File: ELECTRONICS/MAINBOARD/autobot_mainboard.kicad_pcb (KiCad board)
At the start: 4 copper layers, 268 x 112 mm, 164 parts, among them IC1 DW3210, J1 USB_C_Receptacle_USB2.0_16P, J10 Conn_01x05_Socket, J11 Conn_01x01_Socket, J12 Conn_01x02_Pin, J13 Conn_01x01_Socket, J17 Conn_01x02_Pin, J18 Conn_01x02_Pin, J19 Conn_02x05_Odd_Even, J2 Conn_01x01_Socket, J20 Conn_02x05_Odd_Even, J3 Conn_01x01_Socket, J4 Conn_01x02_Socket, J5 Conn_01x01_Socket, J6 Conn_01x01_Socket, J7 Conn_01x03_Pin, J8 Conn_Coaxial, J9 Conn_Coaxial, Q1 DMG1012T, Q2 DMG1012T, Q3 DMG1012T, Q4 DMG1012T, Q5 DMG1012T, SW1 RESET, SW2 BOOT, SW3 SW_Push, U1 TVS1400DRV, U10 VL53L1X, U11 VL53L1X, U12 VL53L1X, U13 BMI270, U14 BMI270, U16 LP5907MFX-3.3, U18 LP5907MFX-3.3, U19 STM32H743VITx, U2 LMR51430XDDCR, U23 LP5907MFX-3.3, U3 LP5907MFX-3.3, U4 TPD2EUSB30A, U7 STM32G031C_4-6-8_Tx, U9 VL53L1X, Y1 TXC 8Y38472012, Y2 25mhz placeholder

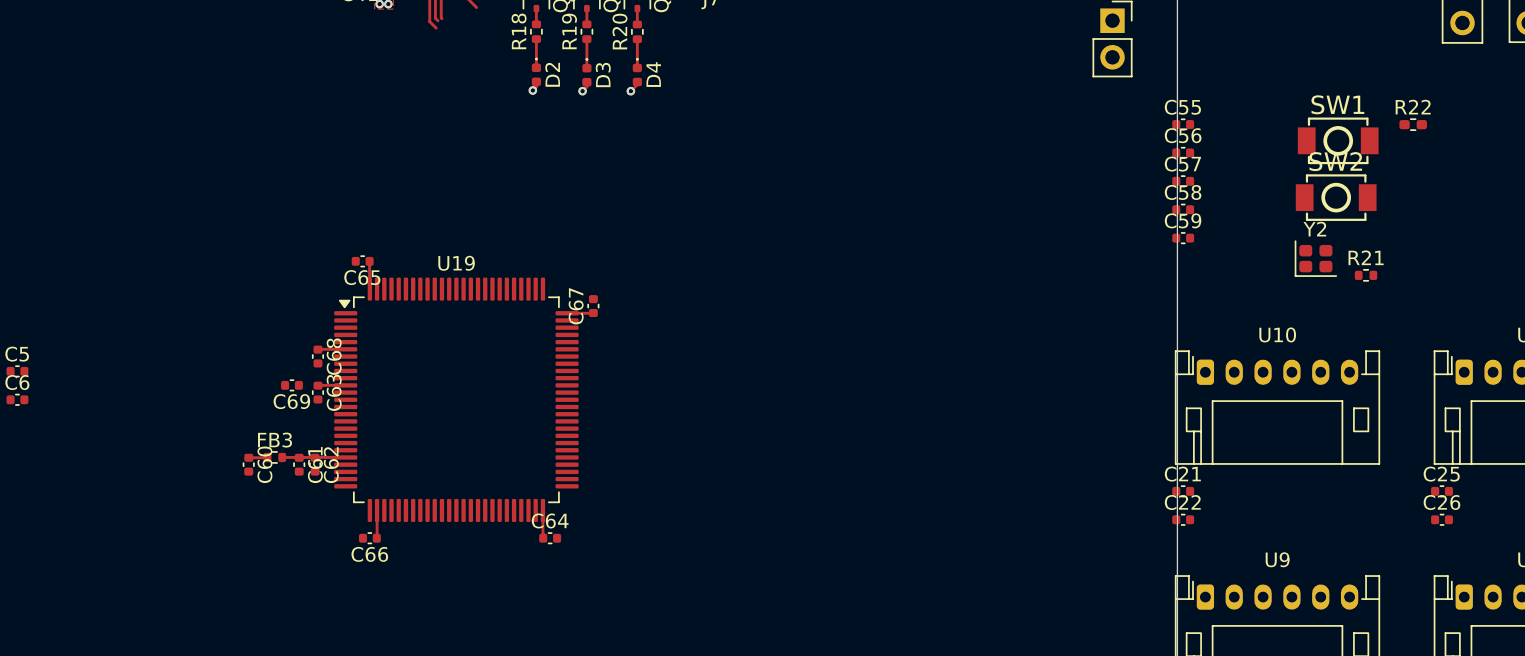
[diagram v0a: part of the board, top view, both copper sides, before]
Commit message: stuff on the h743 prelim route
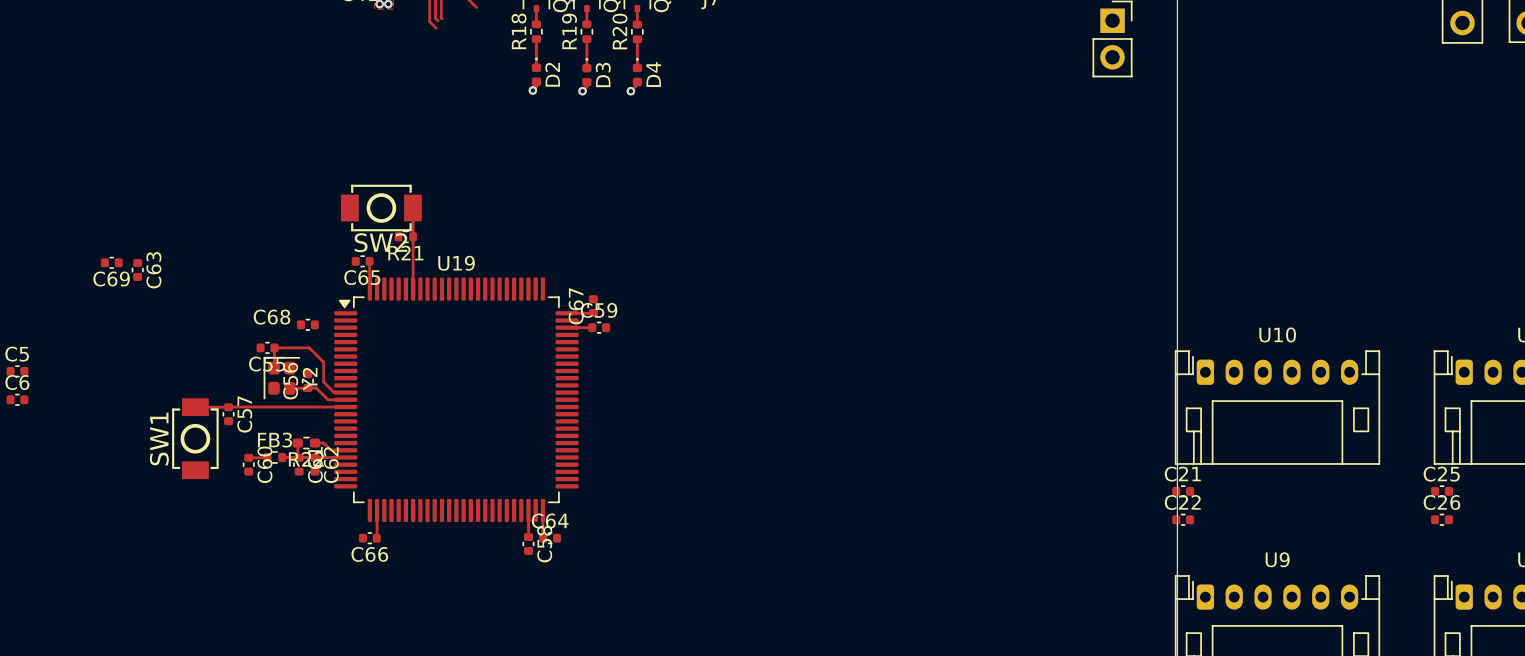
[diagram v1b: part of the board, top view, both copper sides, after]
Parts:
- moved SW1 81.9 mm to (211.9, 82.7), turned to 90 degrees
- moved R22 79.9 mm to (219.6, 83.0), turned to 180 degrees
- moved Y2 72.2 mm to (217.9, 78.5), turned to -90 degrees
- moved C57 68.1 mm to (214.2, 81.0), turned to -90 degrees
- moved R21 66.6 mm to (226.5, 68.7), turned to 180 degrees
- moved SW2 66.2 mm to (224.8, 66.7), turned to 180 degrees
- moved C55 65.4 mm to (216.9, 76.4), turned to 180 degrees
- moved C56 62.7 mm to (219.7, 78.7), turned to 90 degrees
- moved C58 51.0 mm to (235.0, 90.0), turned to -90 degrees
- moved C59 41.0 mm to (239.9, 75.0)
- moved C63 15.1 mm to (207.9, 71.0)
- moved C69 15.1 mm to (206.1, 70.5)
- moved C68 2.31 mm to (219.7, 74.8), turned to 180 degrees
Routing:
- net /STM32H743/NRST: track 0.00 -> 10.4 mm
- net /STM32H743/PH0: track 0.00 -> 8.45 mm
- net /STM32H743/BOOT0: track 0.00 -> 5.63 mm
- net /STM32H743/PH1: track 0.00 -> 4.22 mm
- net +3V3: track 95.7 -> 91.8 mm
- net /STM32H743/VREF: track 0.00 -> 2.34 mm
- net Net-(C58-Pad1): track 0.00 -> 1.84 mm
- net Net-(C59-Pad1): track 0.00 -> 1.74 mm
- net Net-(U19-VDDA): track 4.41 -> 5.47 mm
